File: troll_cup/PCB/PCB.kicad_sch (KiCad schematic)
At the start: 9 parts, among them SW1 SW_Push, SW2 SW_Push, U1 ATtiny85-20P, U2 DFPLAYER MINI

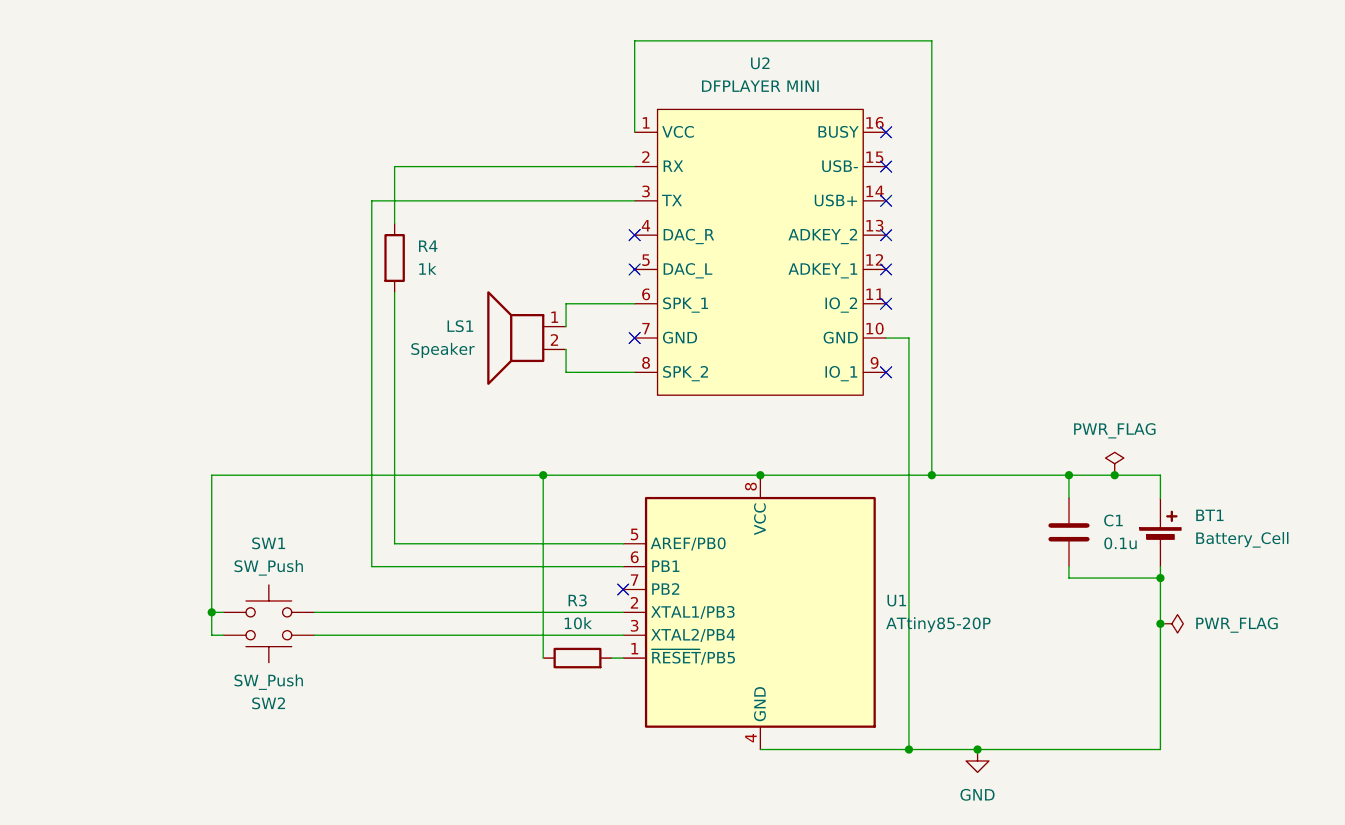
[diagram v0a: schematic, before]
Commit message: Organize schematic
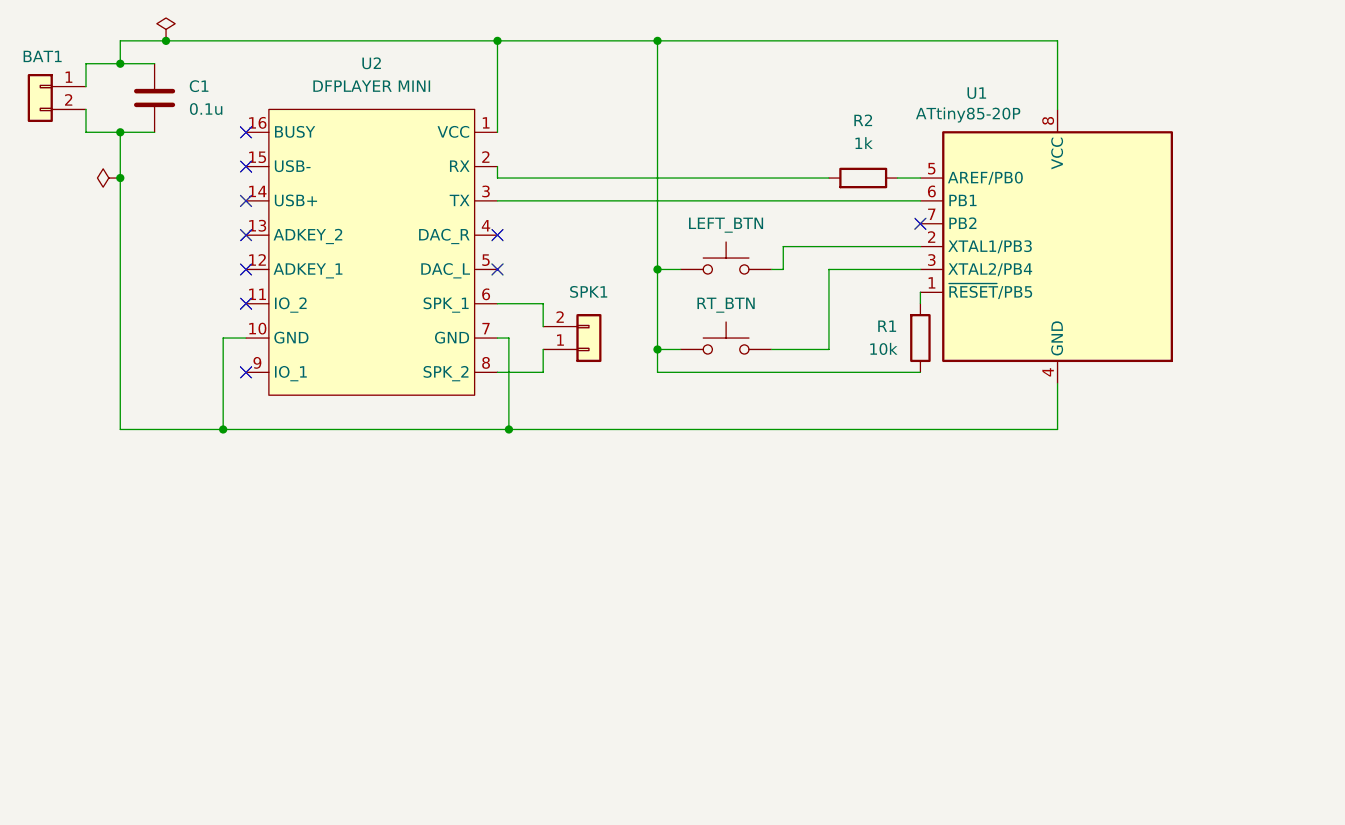
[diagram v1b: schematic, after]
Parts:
- removed BT1: Battery_Cell, symbol Device:Battery_Cell
- removed LS1: Speaker, symbol Device:Speaker
- added BAT1: TO_BATTERY, Connector_JST:JST_PH_S2B-PH-K_1x02_P2.00mm_Horizontal, symbol Connector_Generic:Conn_01x02
- added SPK1: ~, Connector_JST:JST_PH_S2B-PH-K_1x02_P2.00mm_Horizontal, symbol Connector_Generic:Conn_01x02
- C1: footprint (none) -> Capacitor_SMD:C_0603_1608Metric_Pad1.08x0.95mm_HandSolder
- R1: renamed from R3; footprint (none) -> Resistor_SMD:R_0805_2012Metric_Pad1.20x1.40mm_HandSolder
- R2: renamed from R4; footprint (none) -> Resistor_SMD:R_0805_2012Metric_Pad1.20x1.40mm_HandSolder
- SW1: value SW_Push -> LEFT_BTN
- SW2: value SW_Push -> RT_BTN
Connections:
- net GND is gone; now on an unnamed net: C1.1, U1.4 (GND), U2.10 (GND)
- net at C1.2, R1.1, U1.8 (VCC)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: now also SW1.2, SW2.2, BAT1.1 (Pin_1); no longer SW1.1, SW2.1
- net at U1.2 (XTAL1/PB3): now also SW1.1; no longer SW1.2
- net at U1.3 (XTAL2/PB4): now also SW2.1; no longer SW2.2
- net at U1.5 (AREF/PB0): now also R2.1; no longer R2.2
- net at U2.2 (RX): now also R2.2; no longer R2.1
- net at U2.6 (SPK_1): now also SPK1.2 (Pin_2)
- net at U2.8 (SPK_2): now also SPK1.1 (Pin_1)
- net at U2.7 (GND): now also BAT1.2 (Pin_2)
- no-connect marks 11 -> 10
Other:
- moved on the sheet: C1, R1, R2, U1, U2
